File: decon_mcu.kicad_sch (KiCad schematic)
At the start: 5 parts, among them J1 Conn_01x16, J2 Conn_01x16, J3 Conn_01x16, J4 Conn_01x16, U3 STM32F401R_B-C_Tx

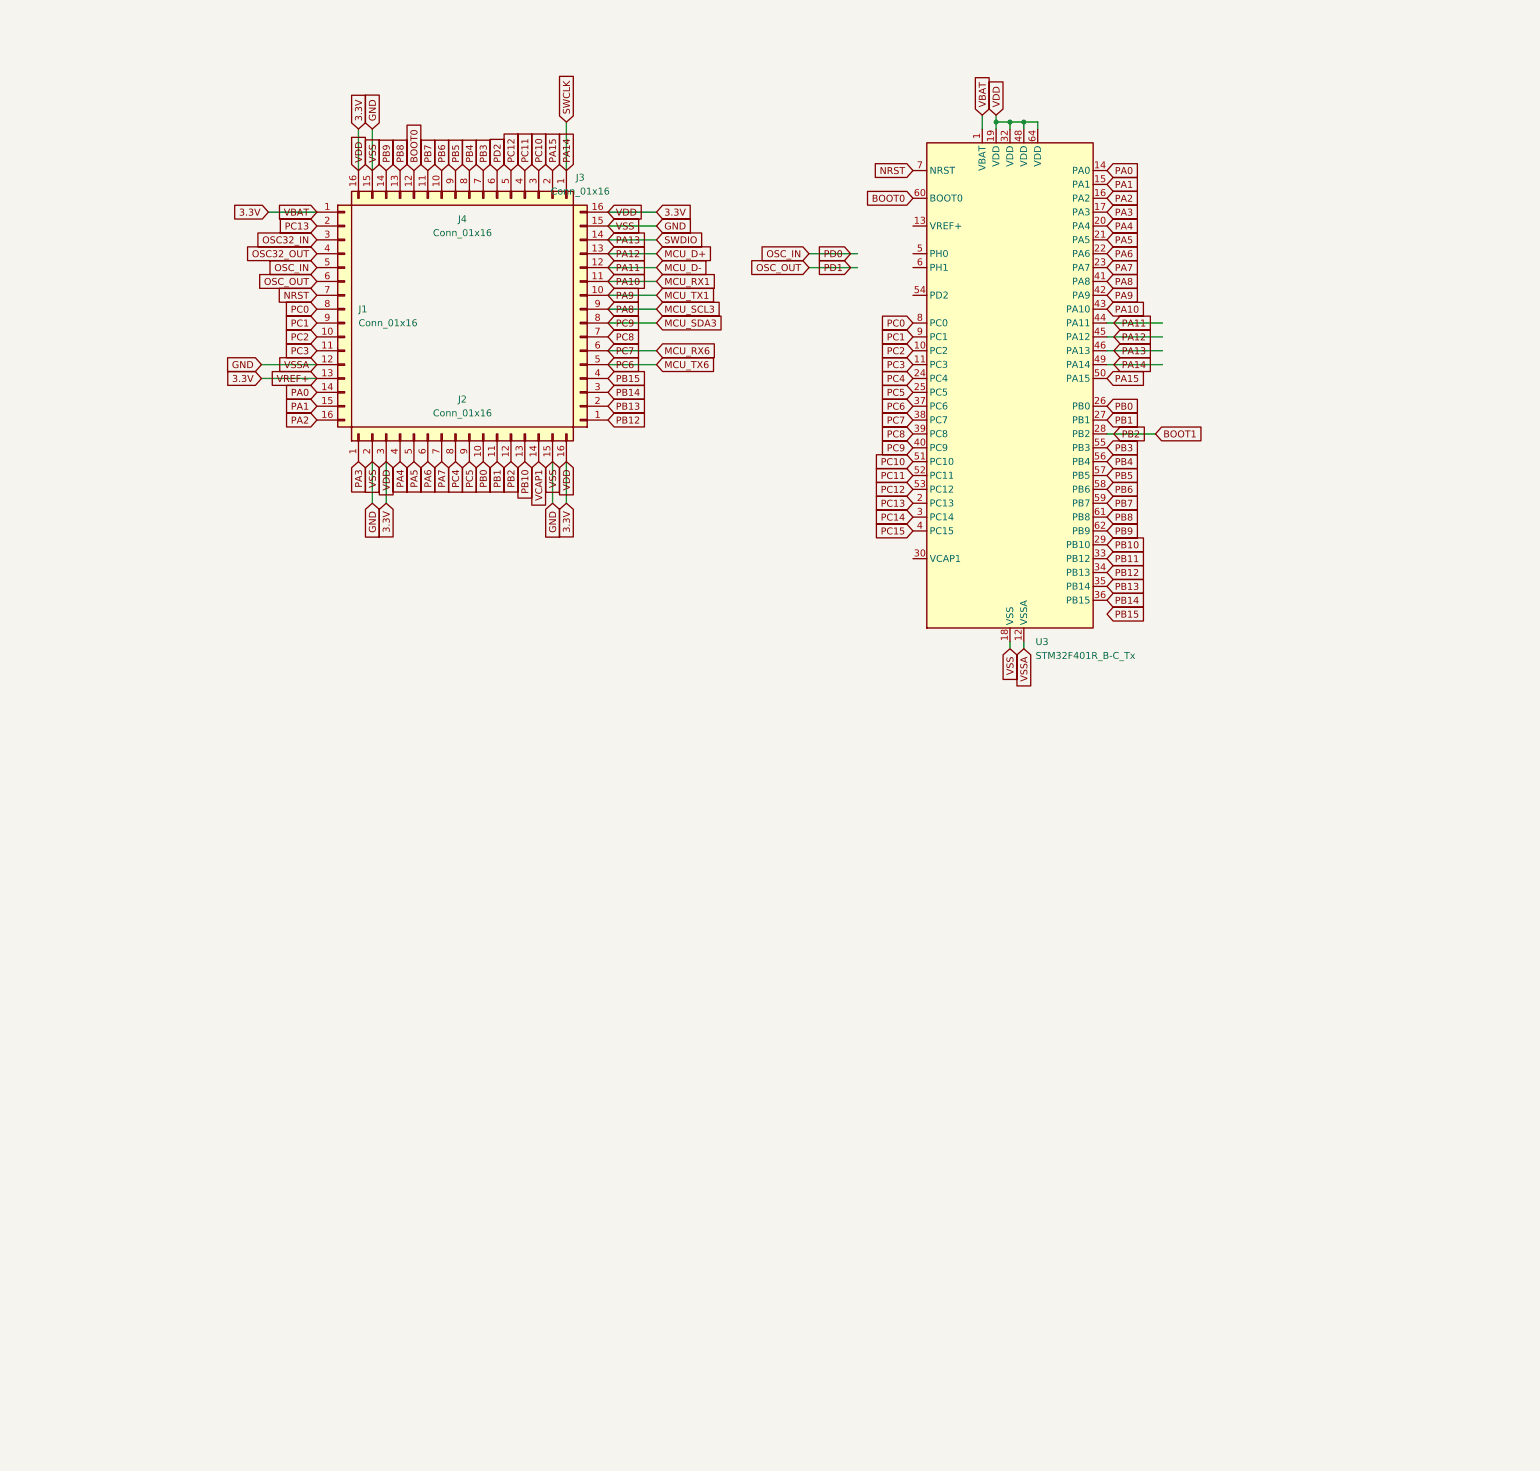
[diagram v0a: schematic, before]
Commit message: new file:   decon_ctrl.pdf
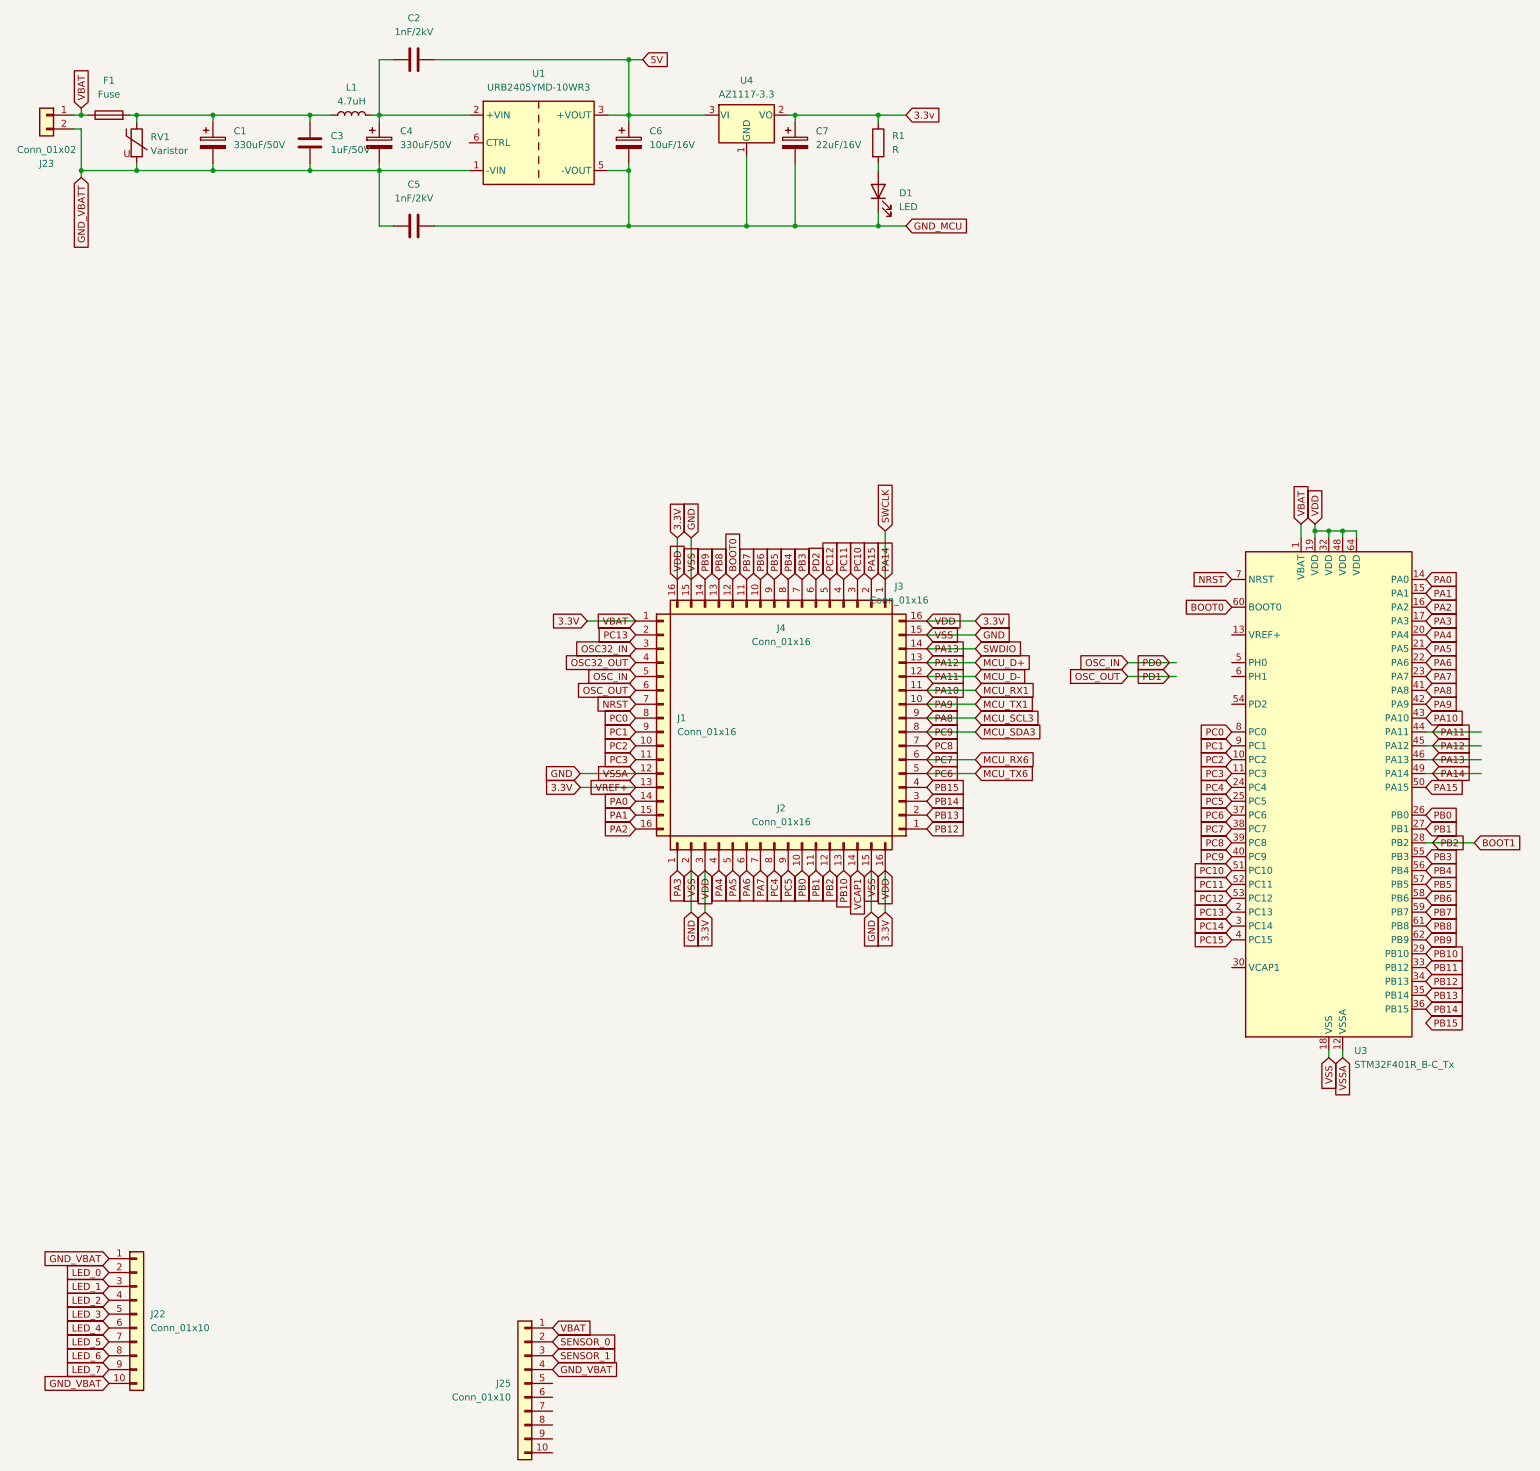
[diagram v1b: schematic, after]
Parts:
- added C1, C4: 330uF/50V, Capacitor_SMD:CP_Elec_10x10.5, symbol Device:C_Polarized
- added C2, C5: 1nF/2kV, Capacitor_THT:C_Disc_D5.0mm_W2.5mm_P5.00mm, symbol Device:C
- added C3: 1uF/50V, Capacitor_SMD:C_0805_2012Metric, symbol Device:C
- added C6: 10uF/16V, Capacitor_SMD:CP_Elec_4x5.4, symbol Device:C_Polarized
- added C7: 22uF/16V, Capacitor_SMD:CP_Elec_4x5.4, symbol Device:C_Polarized
- added D1: LED, LED_SMD:LED_0805_2012Metric, symbol Device:LED
- added F1: Fuse, Fuse:Fuseholder_Clip-5x20mm_Eaton_1A5601-01_Inline_P20.80x6.76mm_D1.70mm_Horizontal, symbol Device:Fuse
- added J22, J25: Conn_01x10, Connector_Phoenix_MC:PhoenixContact_MC_1,5_10-G-3.81_1x10_P3.81mm_Horizontal, symbol Connector_Generic:Conn_01x10
- added J23: Conn_01x02, symbol Connector_Generic:Conn_01x02
- added L1: 4.7uH, Inductor_SMD:L_APV_APH0630, symbol Device:L
- added R1: R, Resistor_SMD:R_0805_2012Metric, symbol Device:R
- added RV1: Varistor, Varistor:RV_Disc_D7mm_W3.4mm_P5mm, symbol Device:Varistor
- added U1: URB2405YMD-10WR3, Son_KiCad_lib:URB2405YMD-10WR3, symbol Son_KiCad_lib:URB2405YMD-10WR3
- added U4: AZ1117-3.3, Package_TO_SOT_SMD:SOT-223-3_TabPin2, symbol Regulator_Linear:AZ1117-3.3
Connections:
- net 3.3V: now also F1.1, J23.1 (Pin_1), J25.1 (Pin_1)
- new net: C2.1, C4.1, L1.2, U1.2 (+VIN)
- new net: C1.1, C3.1, F1.2, L1.1, RV1.1
- new net: D1.2 (A), R1.2
- new net 3.3v: C7.1, R1.1, U4.2 (VO)
- new net 5V: C2.2, C6.1, U1.3 (+VOUT), U4.3 (VI)
- new net GND_MCU: C5.2, C6.2, C7.2, D1.1 (K), U1.5 (-VOUT), U4.1 (GND)
- new net GND_VBAT: J22.1 (Pin_1), J22.10 (Pin_10), J25.4 (Pin_4)
- new net GND_VBATT: C1.2, C3.2, C4.2, C5.1, J23.2 (Pin_2), RV1.2, U1.1 (-VIN)
- new net LED_0: J22.2 (Pin_2)
- new net LED_1: J22.3 (Pin_3)
- new net LED_2: J22.4 (Pin_4)
- new net LED_3: J22.5 (Pin_5)
- new net LED_4: J22.6 (Pin_6)
- new net LED_5: J22.7 (Pin_7)
- new net LED_6: J22.8 (Pin_8)
- new net LED_7: J22.9 (Pin_9)
- new net SENSOR_0: J25.2 (Pin_2)
- new net SENSOR_1: J25.3 (Pin_3)
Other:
- moved on the sheet: J1, J2, J3, J4, U3

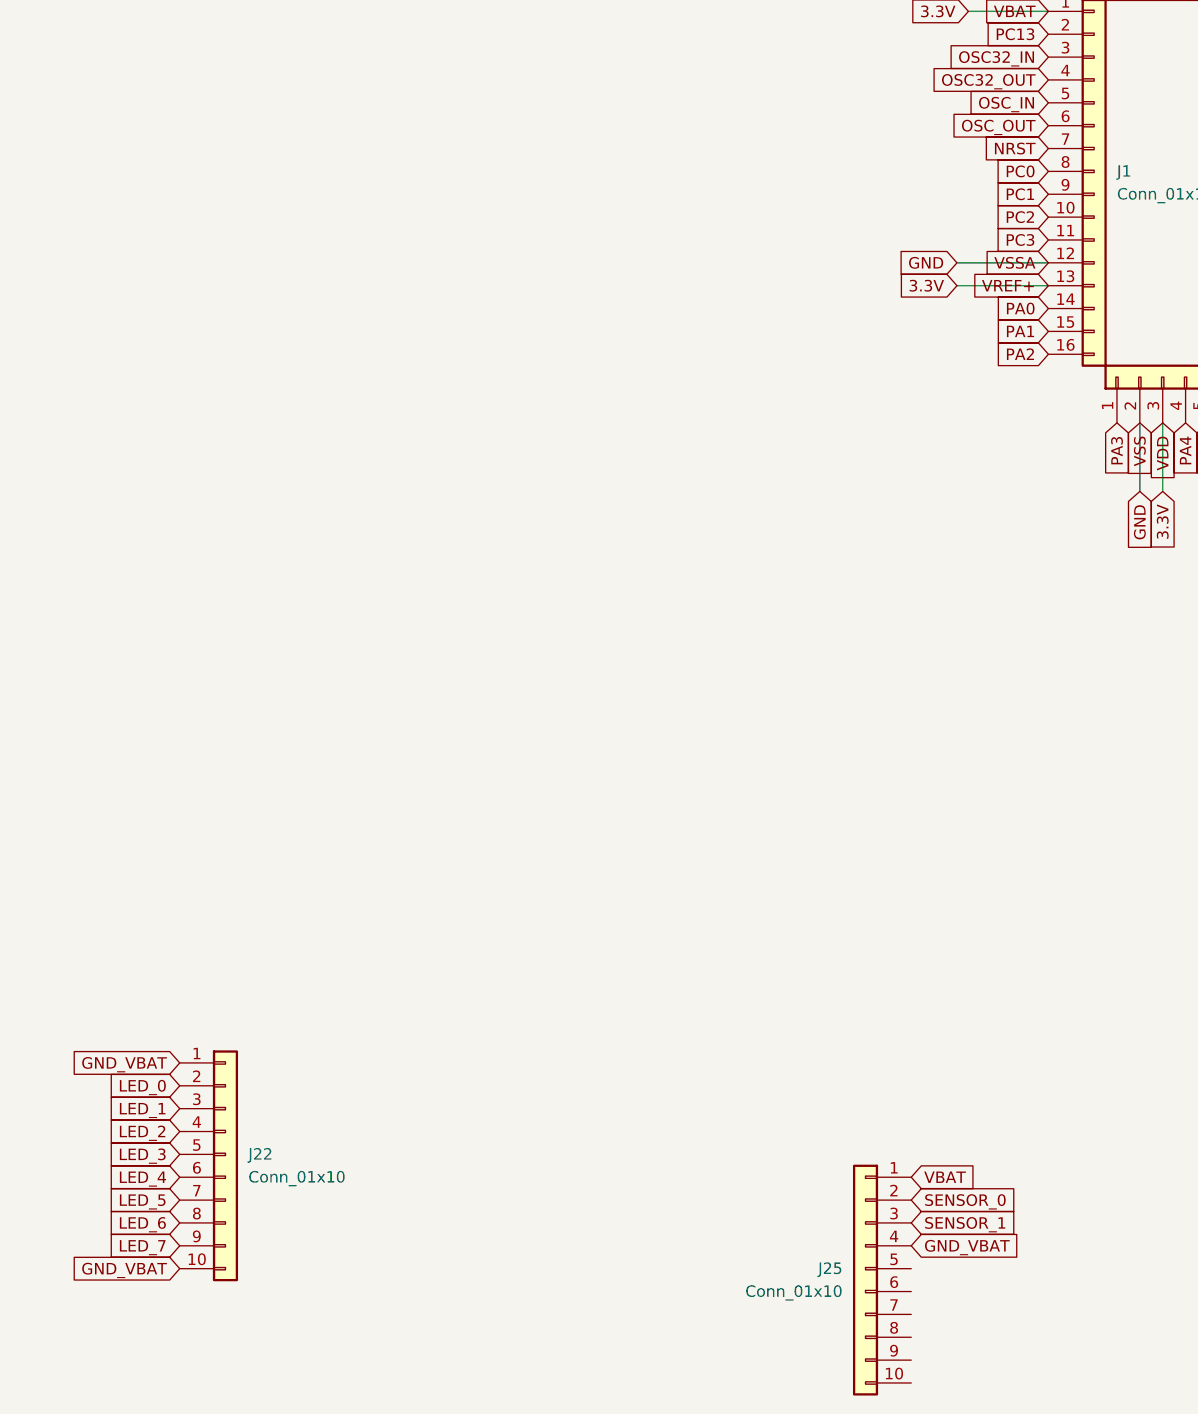
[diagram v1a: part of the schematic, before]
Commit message: modified:   DECON_Ctrl_Panel.kicad_pcb
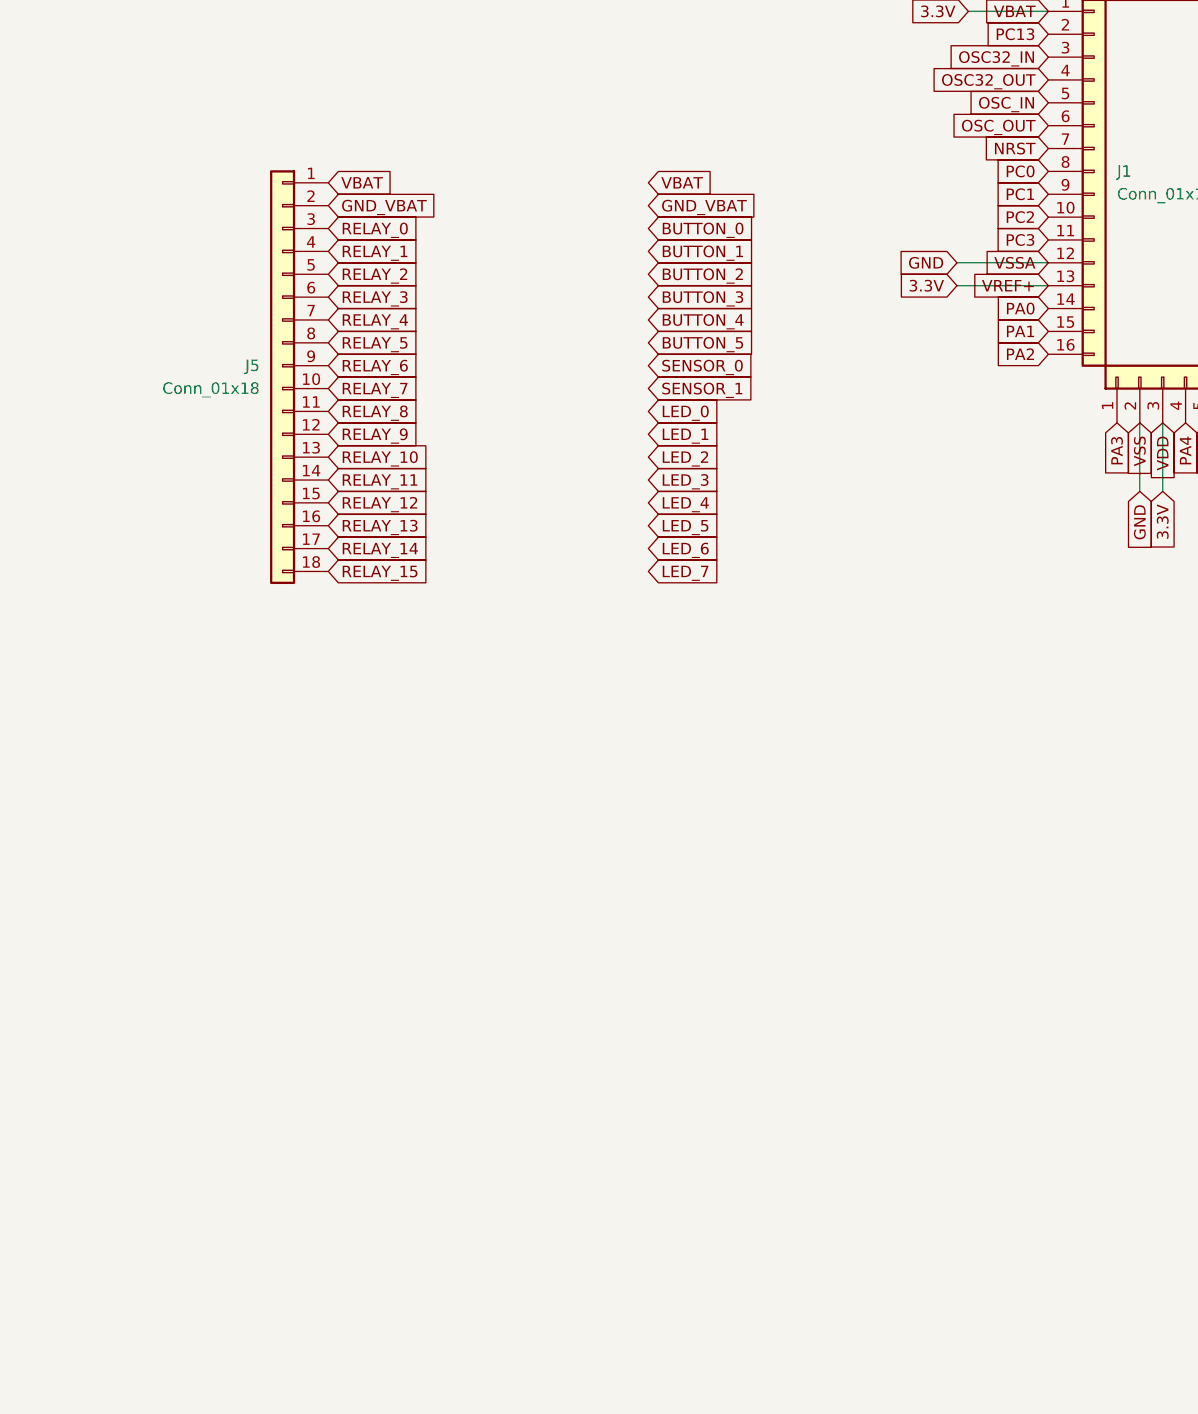
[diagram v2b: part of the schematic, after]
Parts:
- removed J22, J25: Conn_01x10, Connector_Phoenix_MC:PhoenixContact_MC_1,5_10-G-3.81_1x10_P3.81mm_Horizontal, symbol Connector_Generic:Conn_01x10
- added J5: Conn_01x18, symbol Connector_Generic:Conn_01x18
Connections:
- net 3.3V: now also J5.1 (Pin_1)
- net GND_VBAT: now also J5.2 (Pin_2)
- new net RELAY_0: J5.3 (Pin_3)
- new net RELAY_1: J5.4 (Pin_4)
- new net RELAY_10: J5.13 (Pin_13)
- new net RELAY_11: J5.14 (Pin_14)
- new net RELAY_12: J5.15 (Pin_15)
- new net RELAY_13: J5.16 (Pin_16)
- new net RELAY_14: J5.17 (Pin_17)
- new net RELAY_15: J5.18 (Pin_18)
- new net RELAY_2: J5.5 (Pin_5)
- new net RELAY_3: J5.6 (Pin_6)
- new net RELAY_4: J5.7 (Pin_7)
- new net RELAY_5: J5.8 (Pin_8)
- new net RELAY_6: J5.9 (Pin_9)
- new net RELAY_7: J5.10 (Pin_10)
- new net RELAY_8: J5.11 (Pin_11)
- new net RELAY_9: J5.12 (Pin_12)
